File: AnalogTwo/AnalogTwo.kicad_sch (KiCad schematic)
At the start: 22 parts, among them J1 Conn_02x08_Odd_Even, J10 Conn_Coaxial_Small, J11 Conn_Coaxial_Small, J12 Conn_Coaxial_Small, J13 Conn_Coaxial_Small, J14 Conn_Coaxial_Small, J15 Conn_Coaxial_Small, J16 Conn_Coaxial_Small, J2 Conn_02x16_Odd_Even, J25 Conn_Coaxial_Small, J26 Conn_Coaxial_Small, J27 Conn_Coaxial_Small, J28 Conn_Coaxial_Small, J3 Conn_02x20_Odd_Even, J4 Conn_Coaxial_Small, J5 Conn_Coaxial_Small, J6 Conn_Coaxial_Small, J9 Conn_Coaxial_Small

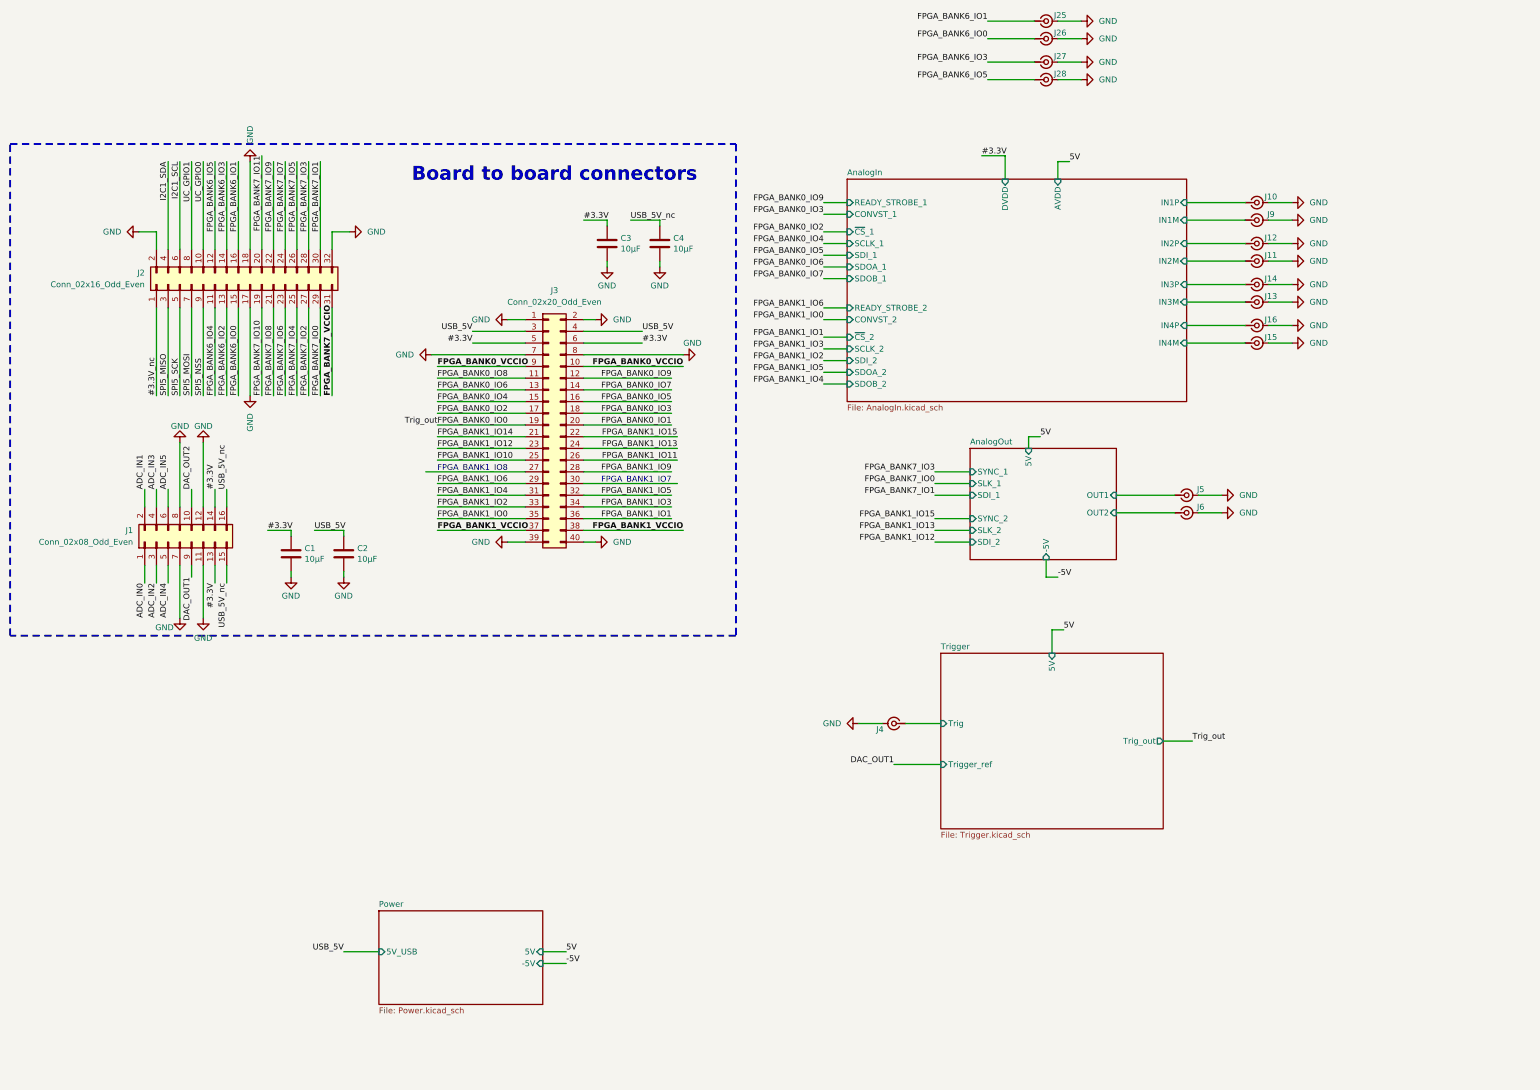
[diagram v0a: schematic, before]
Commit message: AnaloghTwo ready for production
Signed-off-by: Alexis Jeandet <alexis.jeandet@member.fsf.org>
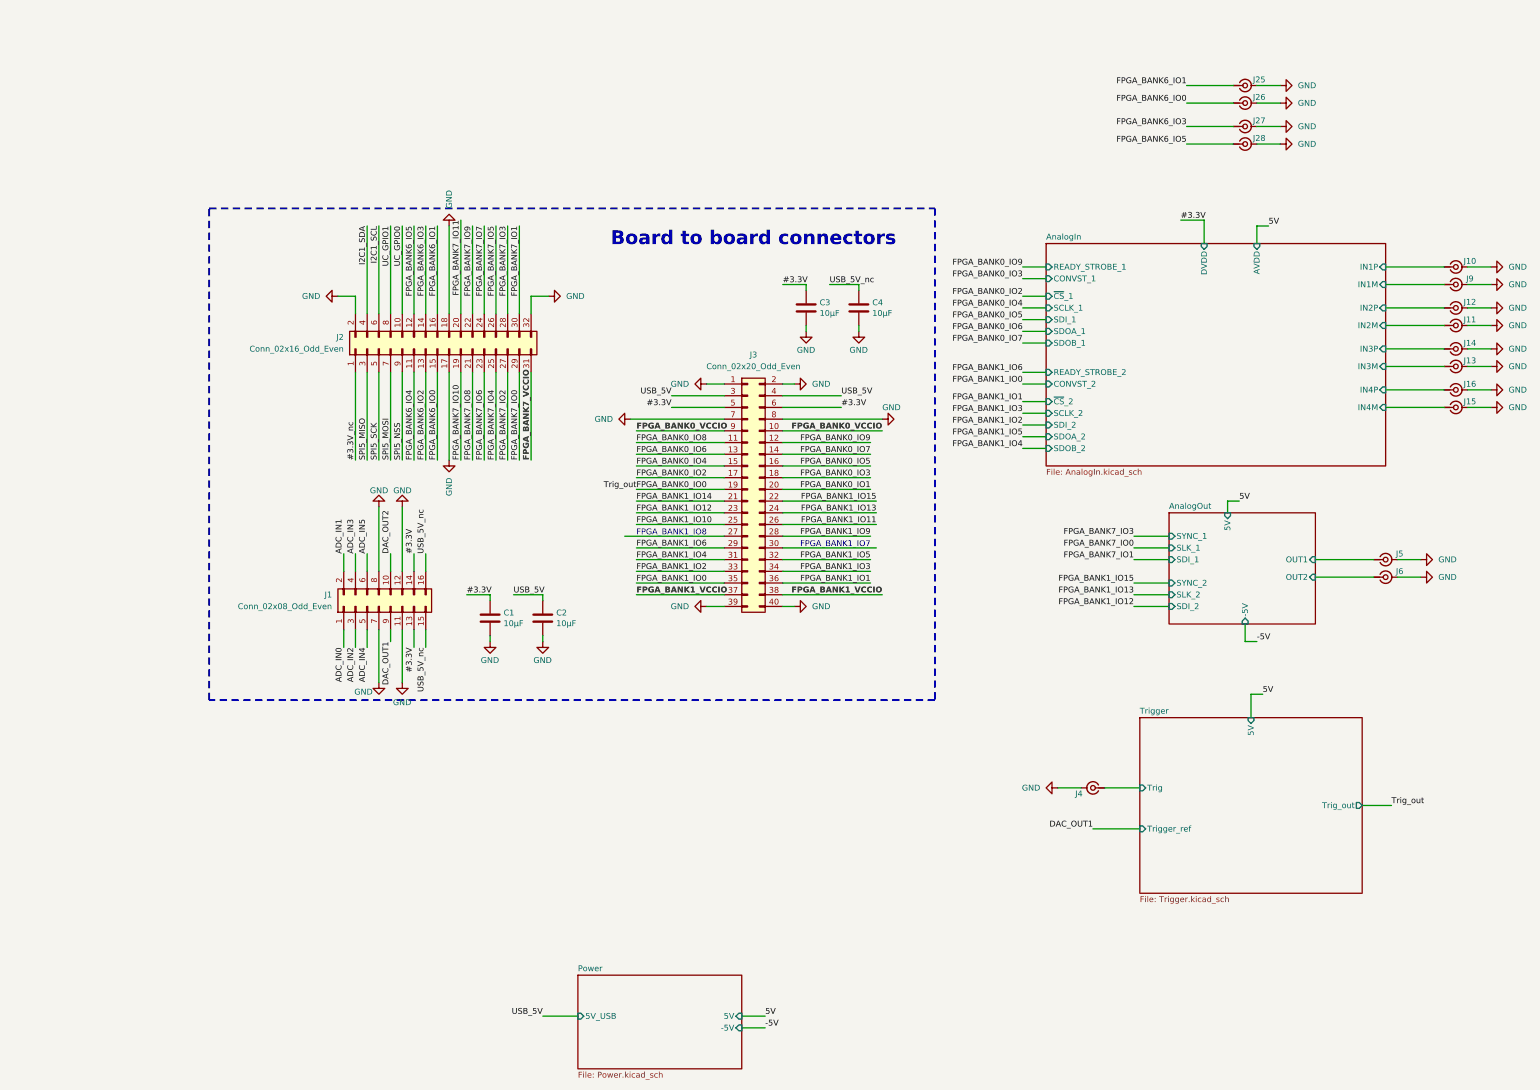
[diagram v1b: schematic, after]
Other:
- moved on the sheet: C1, C2, C3, C4, J1, J10, J11, J12, J13, J14, J15, J16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
